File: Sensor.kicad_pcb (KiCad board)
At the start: 2 copper layers, 49.5 x 49.5 mm, 51 parts, among them IC1 STM32L051K8T6, P1 CONN_02X04, P3 CONN_02X04, P4 CONN_01X04, P5 CONN_01X02, Q1 AO3401, Q2 AO3401, Q4 AO3401, Q5 AO3401, SW1 SW_PUSH, U1 PIR, U2 MCP6004, U3 EPL3015, U4 TPS61222

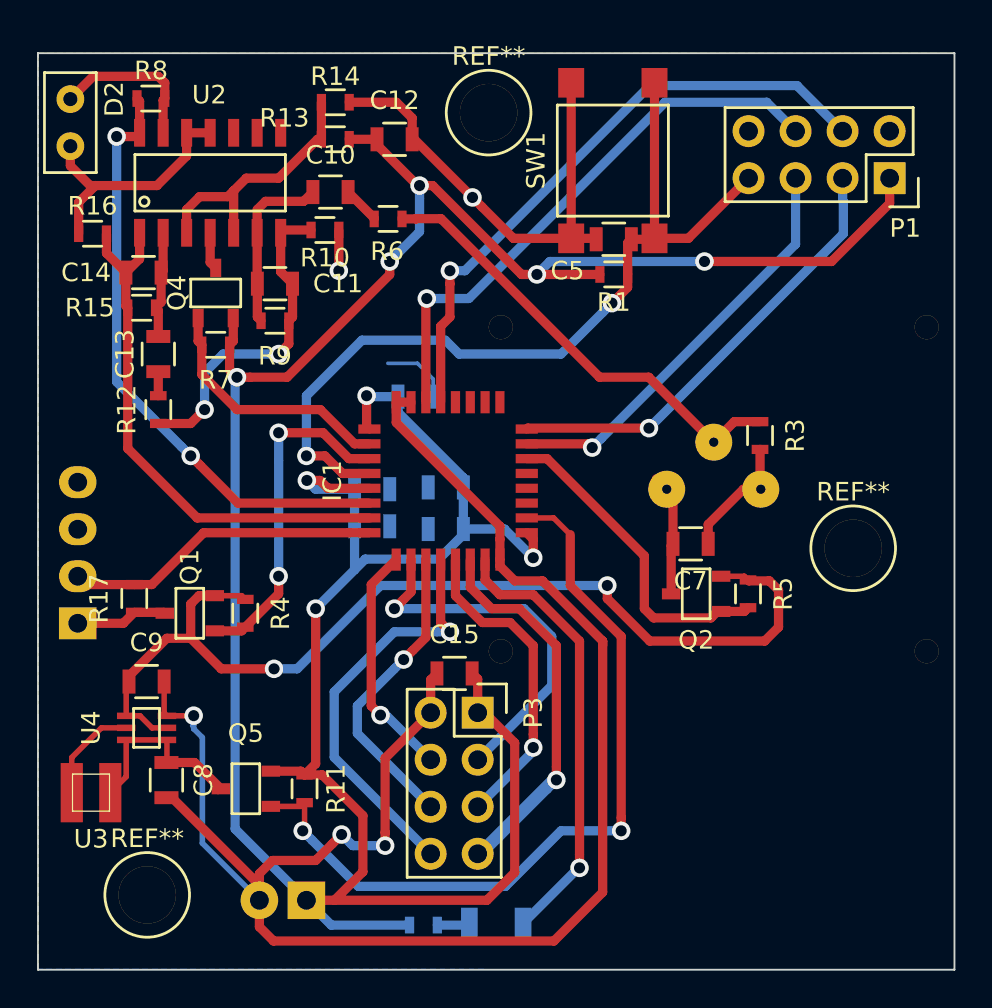
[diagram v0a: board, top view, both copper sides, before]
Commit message: Finish schematic, assign all footprints for V3
Signed-off-by: pluyckx <philip.luyckx@gmail.com>
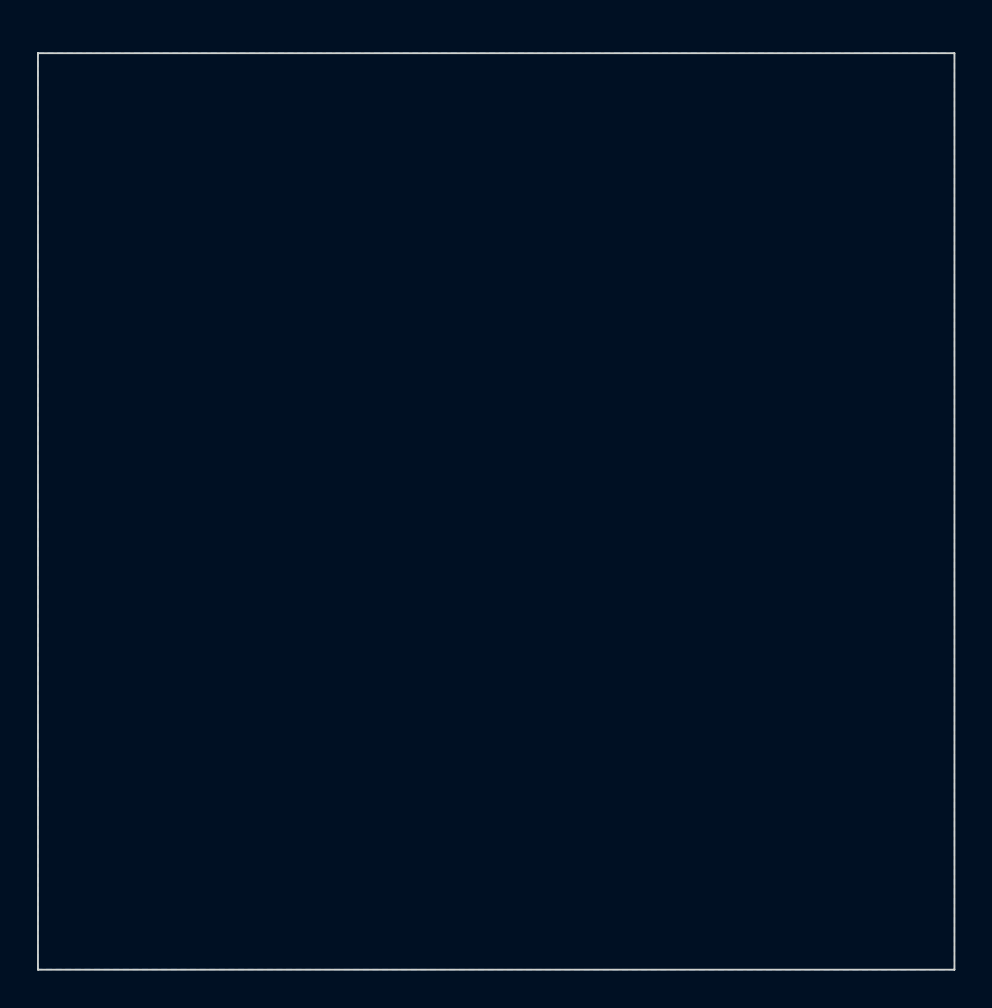
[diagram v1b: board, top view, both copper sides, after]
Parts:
- removed C1, C10, C13, C7, C8, C9: 10uF, Resistors_SMD:R_0805
- removed C11, C12, C14, C15, C3, C4, C5, C6: 100nF, Resistors_SMD:R_0805
- removed C2: 1uF, Resistors_SMD:R_0805
- removed D1: LED, Resistors_SMD:R_1206
- removed D2: PhotoDiode, CustomModules:PD638C
- removed IC1: STM32L051K8T6, STM32:STM32L051-LQFP32
- removed P1, P3: CONN_02X04, Socket_Strips:Socket_Strip_Straight_2x04
- removed P4: CONN_01X04, Socket_Strips:Socket_Strip_Angled_1x04
- removed P5: CONN_01X02, Socket_Strips:Socket_Strip_Straight_1x02
- removed Q1, Q2, Q4, Q5: AO3401, CustomSmd:SOT23
- removed R1, R13, R14, R3: 100k, Resistors_SMD:R_0603
- removed R10, R12, R16, R6: 10k, Resistors_SMD:R_0603
- removed R11: 47k, Resistors_SMD:R_0603
- removed R15, R9: 1M, Resistors_SMD:R_0603
- removed R17: 1k, Resistors_SMD:R_0603
- removed R2: 475, Resistors_SMD:R_0603
- removed R4, R5, R7: 47.5k, Resistors_SMD:R_0603
- removed R8: 3600, Resistors_SMD:R_0603
- removed REF** (x3): 1pin, Connect:1pin
- removed SW1: SW_PUSH, CustomSmd:MicroSwitch_6x6mm
- removed U1: PIR, CustomModules:PIR
- removed U2: MCP6004, CustomSmd:SOIC-14
- removed U3: EPL3015, CustomInductors:EPL3015
- removed U4: TPS61222, DC_DC_Converters:TPS6122x
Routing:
- net +BATT: track 177.1 -> 0.00 mm, vias 9 -> 0
- net GND: track 150.0 -> 0.00 mm, vias 5 -> 0
- net +5V: track 55.6 -> 0.00 mm, vias 2 -> 0
- net MCU_RST: track 46.2 -> 0.00 mm, vias 2 -> 0
- net Enable5V: track 43.0 -> 0.00 mm, vias 2 -> 0
- net UART_TX: track 33.7 -> 0.00 mm, vias 1 -> 0
- net ADC_Light: track 32.8 -> 0.00 mm, vias 2 -> 0
- net UART_RX: track 30.6 -> 0.00 mm, vias 1 -> 0
- net ADC_Motion: track 29.1 -> 0.00 mm
- net RF_IRQ: track 26.5 -> 0.00 mm, vias 1 -> 0
- net Motion_Out: track 24.8 -> 0.00 mm
- net SWDCLK: track 24.5 -> 0.00 mm, vias 1 -> 0
- net MCU_LED: track 24.1 -> 0.00 mm, vias 1 -> 0
- net SWDIO: track 22.7 -> 0.00 mm, vias 1 -> 0
- net SPI_RF_MISO: track 22.6 -> 0.00 mm, vias 1 -> 0
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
